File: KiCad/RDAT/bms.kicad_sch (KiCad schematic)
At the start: 29 parts, among them Q1 NMOS, Q2 NMOS, U3 BQ7791500PWT, U4 BQ34Z100PWR-R2

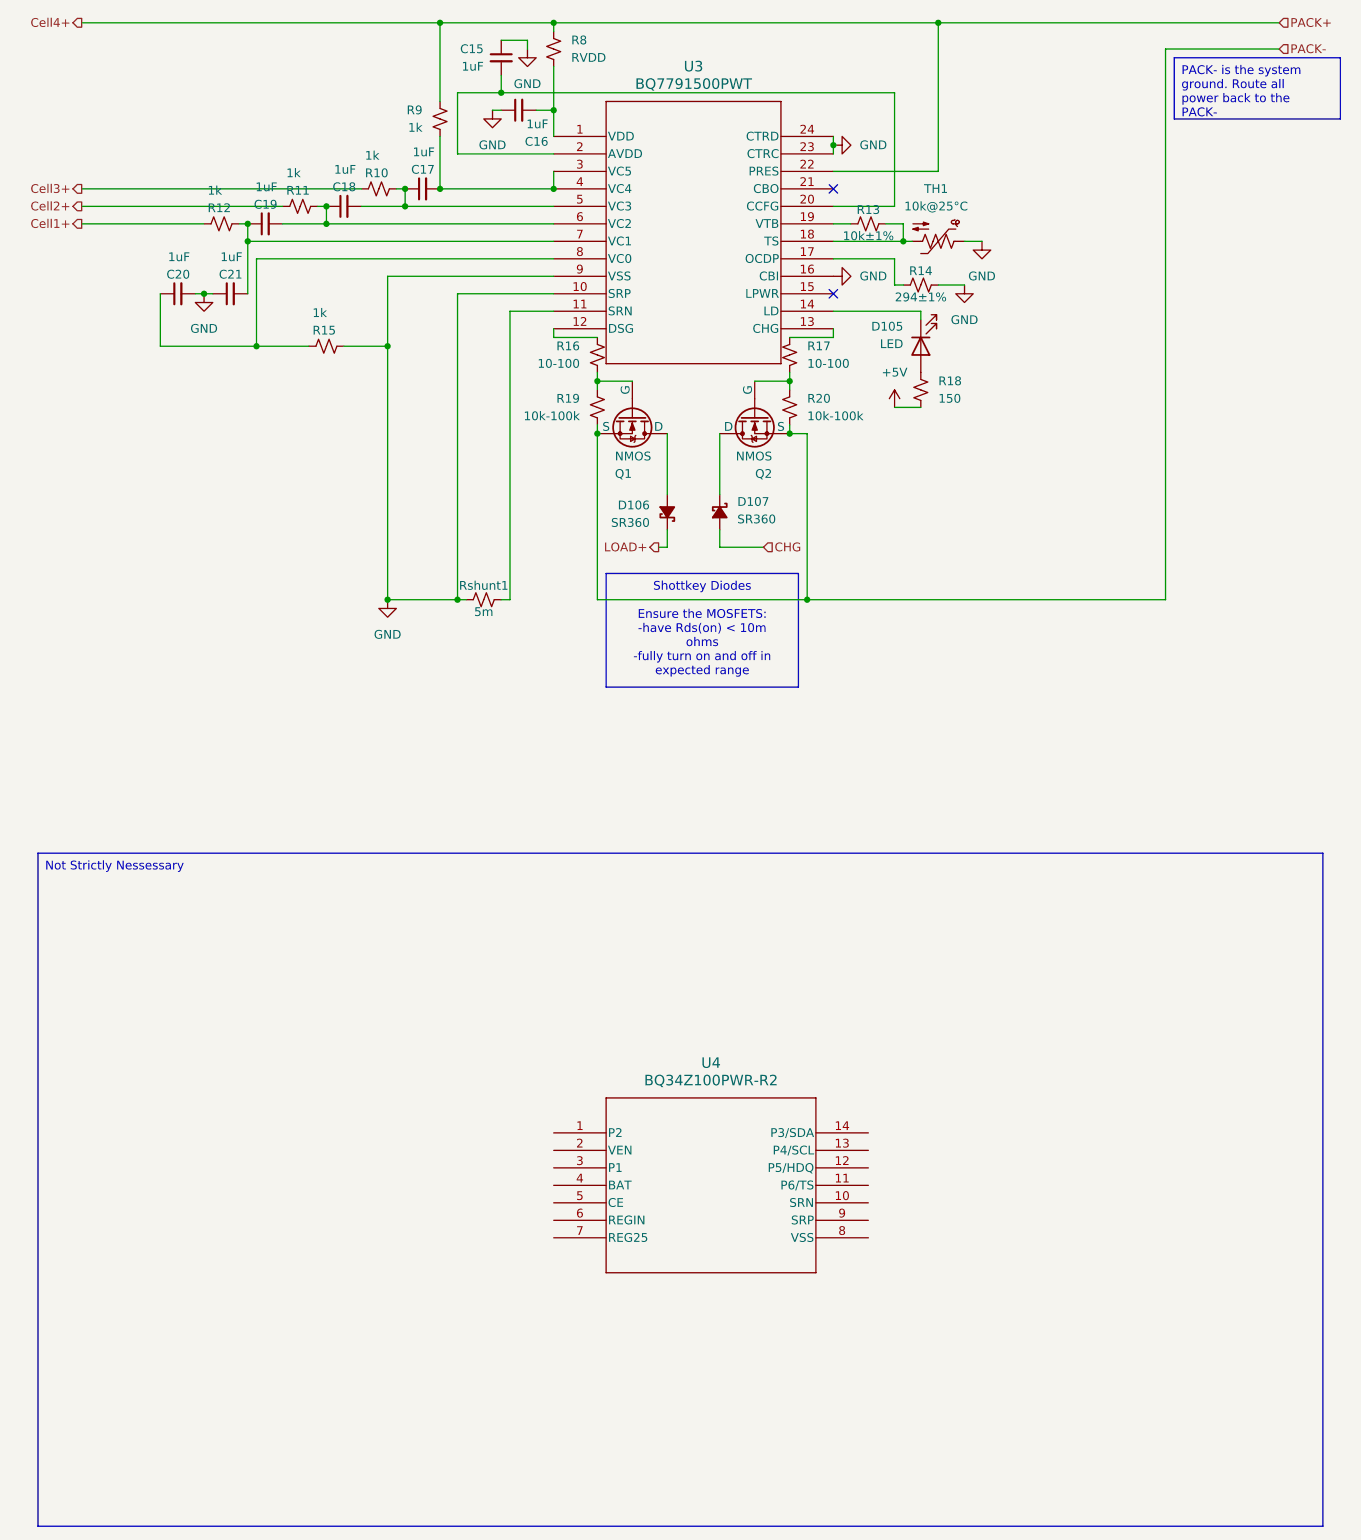
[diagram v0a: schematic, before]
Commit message: added volage stuffs
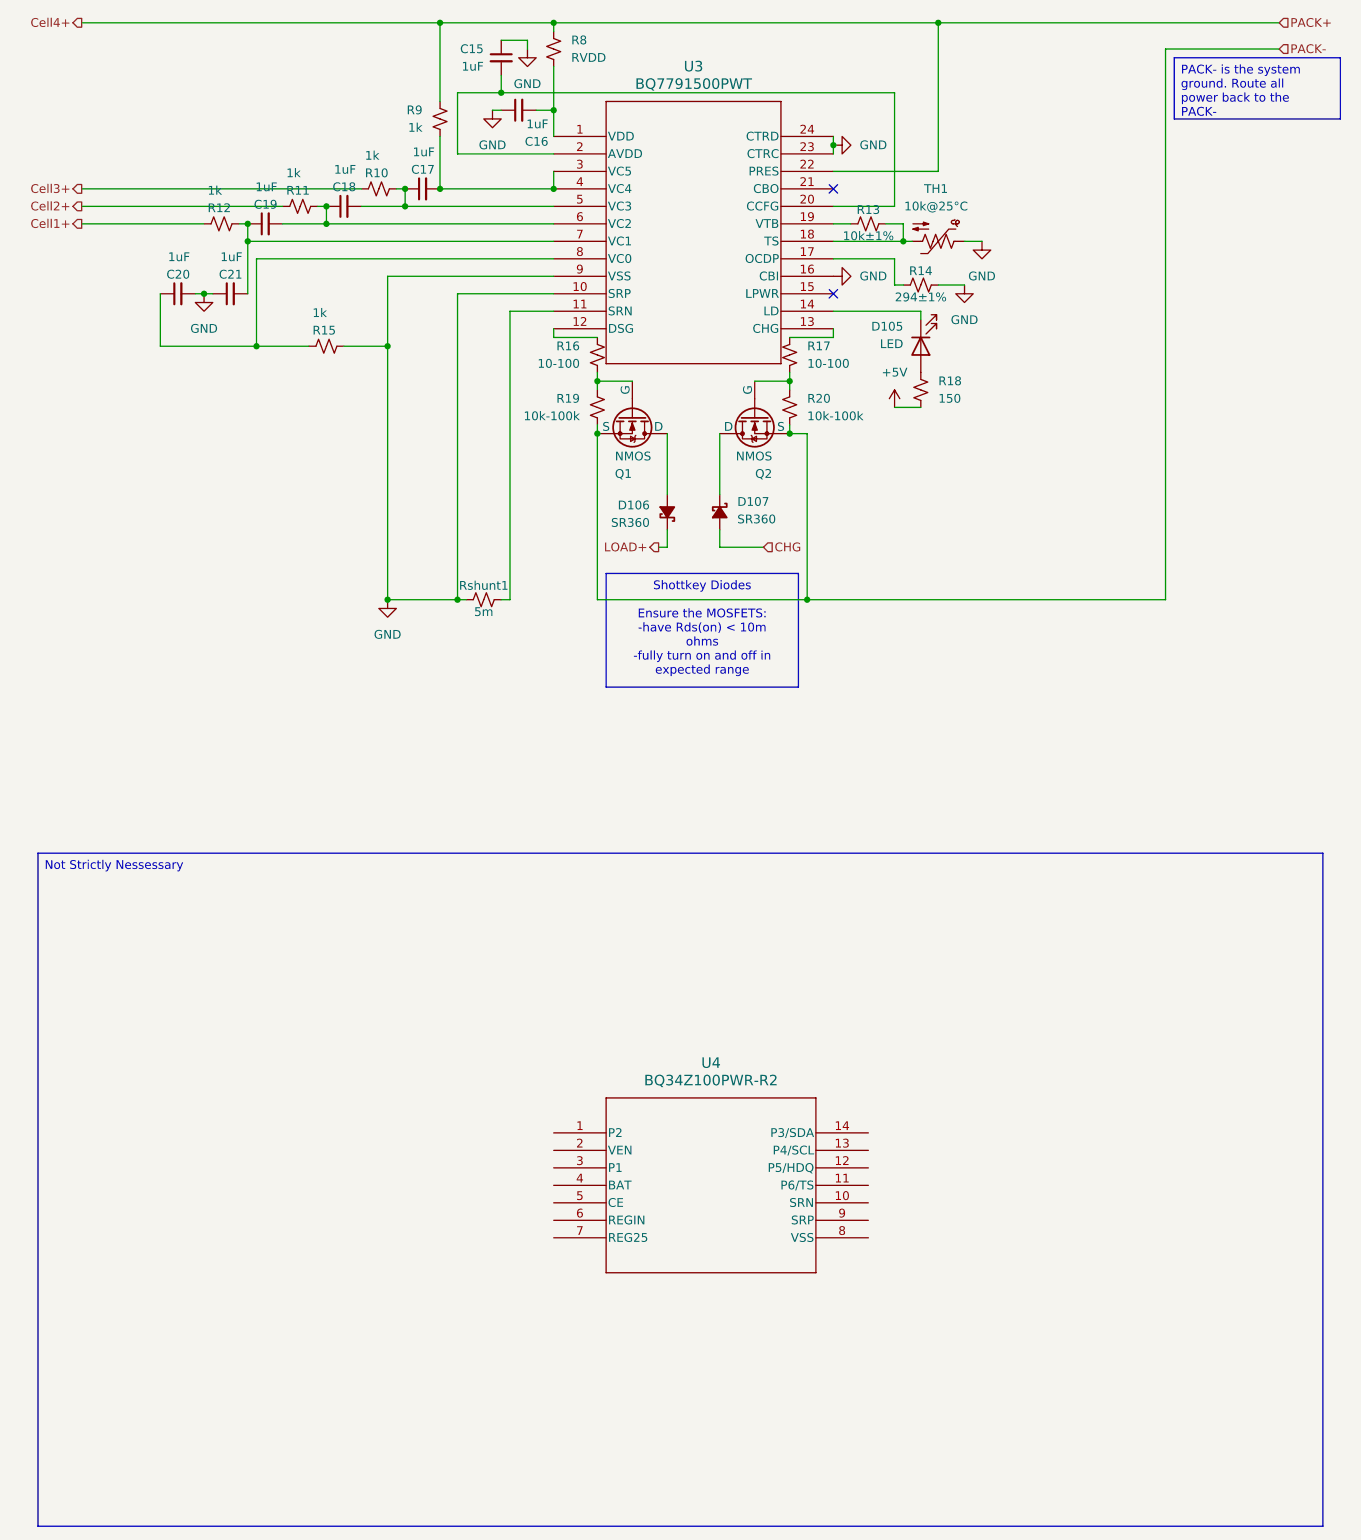
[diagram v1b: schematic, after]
